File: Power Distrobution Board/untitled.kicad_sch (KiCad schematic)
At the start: 4 parts, among them J3 0768250004, K3 AZ2150-1A-12DEF

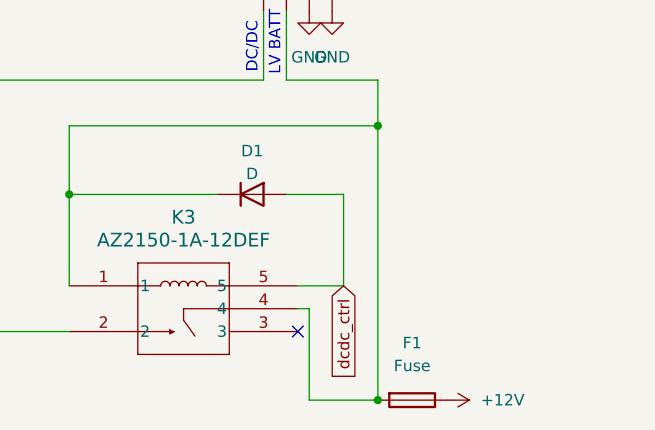
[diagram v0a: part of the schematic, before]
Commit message: changes after cdr
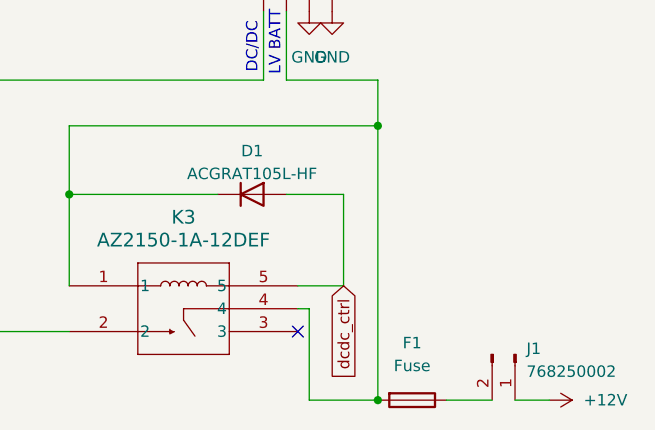
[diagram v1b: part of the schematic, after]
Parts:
- added J1: 768250002, Connector_Molex:Molex_Mega-Fit_76825-0002_2x01_P5.70mm_Horizontal, symbol Connector:Conn_01x02_Pin
- D1: value D -> ACGRAT105L-HF
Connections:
- net +12V: now also J1.1 (Pin_1); no longer F1.1
- new net: F1.1, J1.2 (Pin_2)
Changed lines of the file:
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@@
+	(wire
+		(pts
+			(xy 74.93 74.93) (xy 80.01 74.93)
+		)
+		(stroke
+			(width 0)
+			(type default)
+		)
+	)
 	(wire
 		(pts
@@
 		(pts
 			(xy 59.69 74.93) (xy 67.31 74.93)
+		)
+		(stroke
+			(width 0)
+			(type default)
+		)
+	)
+	(wire
+		(pts
+			(xy 82.55 74.93) (xy 86.36 74.93)
 		)
 		(stroke
@@
 		)
 	)
+	(netclass_flag ""
+		(length 2.54)
+		(shape round)
+		(at 77.47 74.93 180)
+		(fields_autoplaced yes)
+		(effects
+			(font
+				(size 1.27 1.27)
+			)
+			(justify right bottom)
+		)
+		(property "Netclass" "20a"
+			(at 78.1685 77.47 0)
+			(effects
+				(font
+					(size 1.27 1.27)
+					(italic yes)
+				)
+				(justify left)
+			)
+		)
+	)
 	(symbol
 		(lib_id "power:GND")
@@
 	)
 	(symbol
+		(lib_id "Connector:Conn_01x02_Pin")
+		(at 82.55 69.85 270)
+		(unit 1)
+		(exclude_from_sim no)
+		(in_bom yes)
+		(on_board yes)
+		(dnp no)
+		(fields_autoplaced yes)
+		(property "Reference" "J1"
+			(at 83.82 69.2149 90)
+			(effects
+				(font
+					(size 1.27 1.27)
+				)
+				(justify left)
+			)
+		)
+		(property "Value" "768250002"
+			(at 83.82 71.7549 90)
+			(effects
+				(font
+					(size 1.27 1.27)
+				)
+				(justify left)
+			)
+		)
+		(property "Footprint" "Connector_Molex:Molex_Mega-Fit_76825-0002_2x01_P5.70mm_Horizontal"
+			(at 82.55 69.85 0)
+			(effects
+				(font
+					(size 1.27 1.27)
+				)
+				(hide yes)
+			)
+		)
+		(property "Datasheet" "https://mm.digikey.com/Volume0/opasdata/d220001/medias/docus/1100/Mega-Fit_Power_Conn.pdf"
+			(at 82.55 69.85 0)
+			(effects
+				(font
+					(size 1.27 1.27)
+				)
+				(hide yes)
+			)
+		)
+		(property "Description" "Generic connector, single row, 01x02, script generated"
+			(at 82.55 69.85 0)
+			(effects
+				(font
+					(size 1.27 1.27)
+				)
+				(hide yes)
+			)
+		)
+		(pin "2"
+		)
+		(pin "1"
+		)
+		(instances
+			(project ""
+				(path "/cd827802-ab32-49ad-ad84-bccf81c569e7/5e60819f-ad8d-4ea9-981f-2629d0d45dd9"
+					(reference "J1")
+					(unit 1)
+				)
+			)
+		)
+	)
+	(symbol
 		(lib_id "AZ2150:AZ2150-1A-12DEF")
 		(at 33.02 62.23 0)
@@
 			)
 		)
-		(property "Value" "D"
+		(property "Value" "ACGRAT105L-HF"
 			(at 53.34 49.784 0)
 			(effects
@@
 	(symbol
 		(lib_id "power:+12V")
-		(at 74.93 74.93 270)
+		(at 86.36 74.93 270)
 		(unit 1)
 		(exclude_from_sim no)
@@
 		(fields_autoplaced yes)
 		(property "Reference" "#PWR07"
-			(at 71.12 74.93 0)
+			(at 82.55 74.93 0)
 			(effects
 				(font
@@
 		)
 		(property "Value" "+12V"
-			(at 78.74 74.9299 90)
+			(at 90.17 74.9299 90)
 			(effects
 				(font
@@
 		)
 		(property "Footprint" ""
-			(at 74.93 74.93 0)
+			(at 86.36 74.93 0)
 			(effects
 				(font
@@
 		)
 		(property "Datasheet" ""
-			(at 74.93 74.93 0)
+			(at 86.36 74.93 0)
 			(effects
 				(font
@@
 		)
 		(property "Description" "Power symbol creates a global label with name \"+12V\""
-			(at 74.93 74.93 0)
-			(effects
-				(font
+			(at 86.36 74.93 0)
+			(effects
+				(font

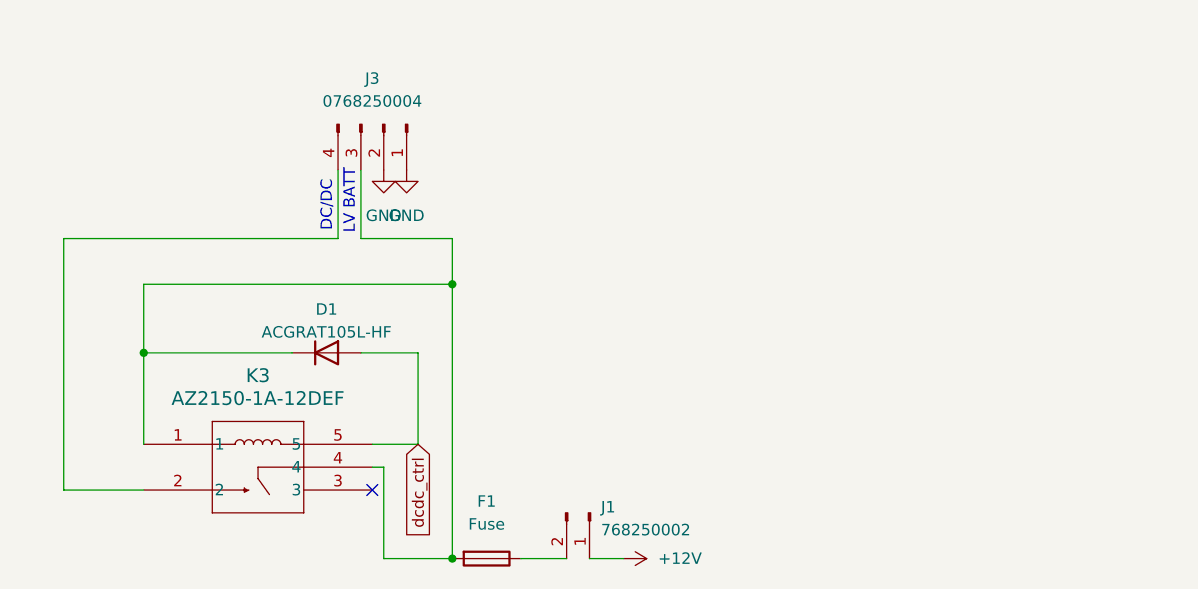
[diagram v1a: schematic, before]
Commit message: even newer changes
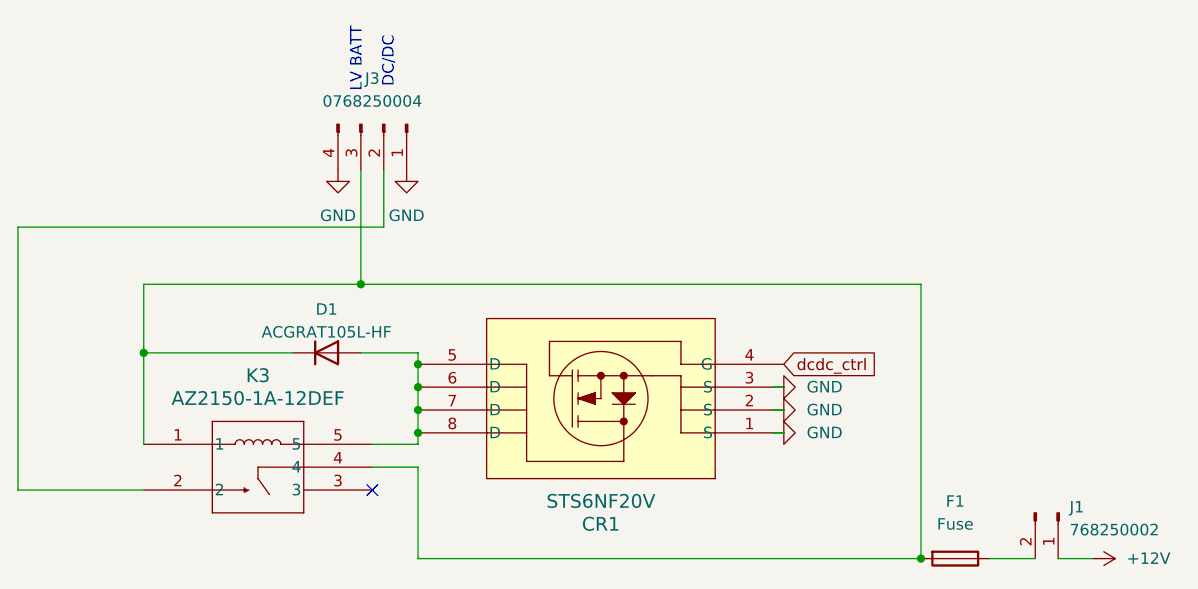
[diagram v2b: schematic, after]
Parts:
- added CR1: STS6NF20V, Package_SO:SOIC-8_3.9x4.9mm_P1.27mm, symbol FS_3_Global_Symbol_Library:STS6NF20V
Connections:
- net GND: now also J3.4 (Pin_4), CR1.1 (S), CR1.2 (S), CR1.3 (S); no longer J3.2 (Pin_2)
- net dcdc_ctrl: now also CR1.4 (G); no longer D1.2 (A), K3.5
- net at K3.2: now also J3.2 (Pin_2); no longer J3.4 (Pin_4)
- new net: CR1.5 (D), CR1.6 (D), CR1.7 (D), CR1.8 (D), D1.2 (A), K3.5
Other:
- moved on the sheet: F1, J1

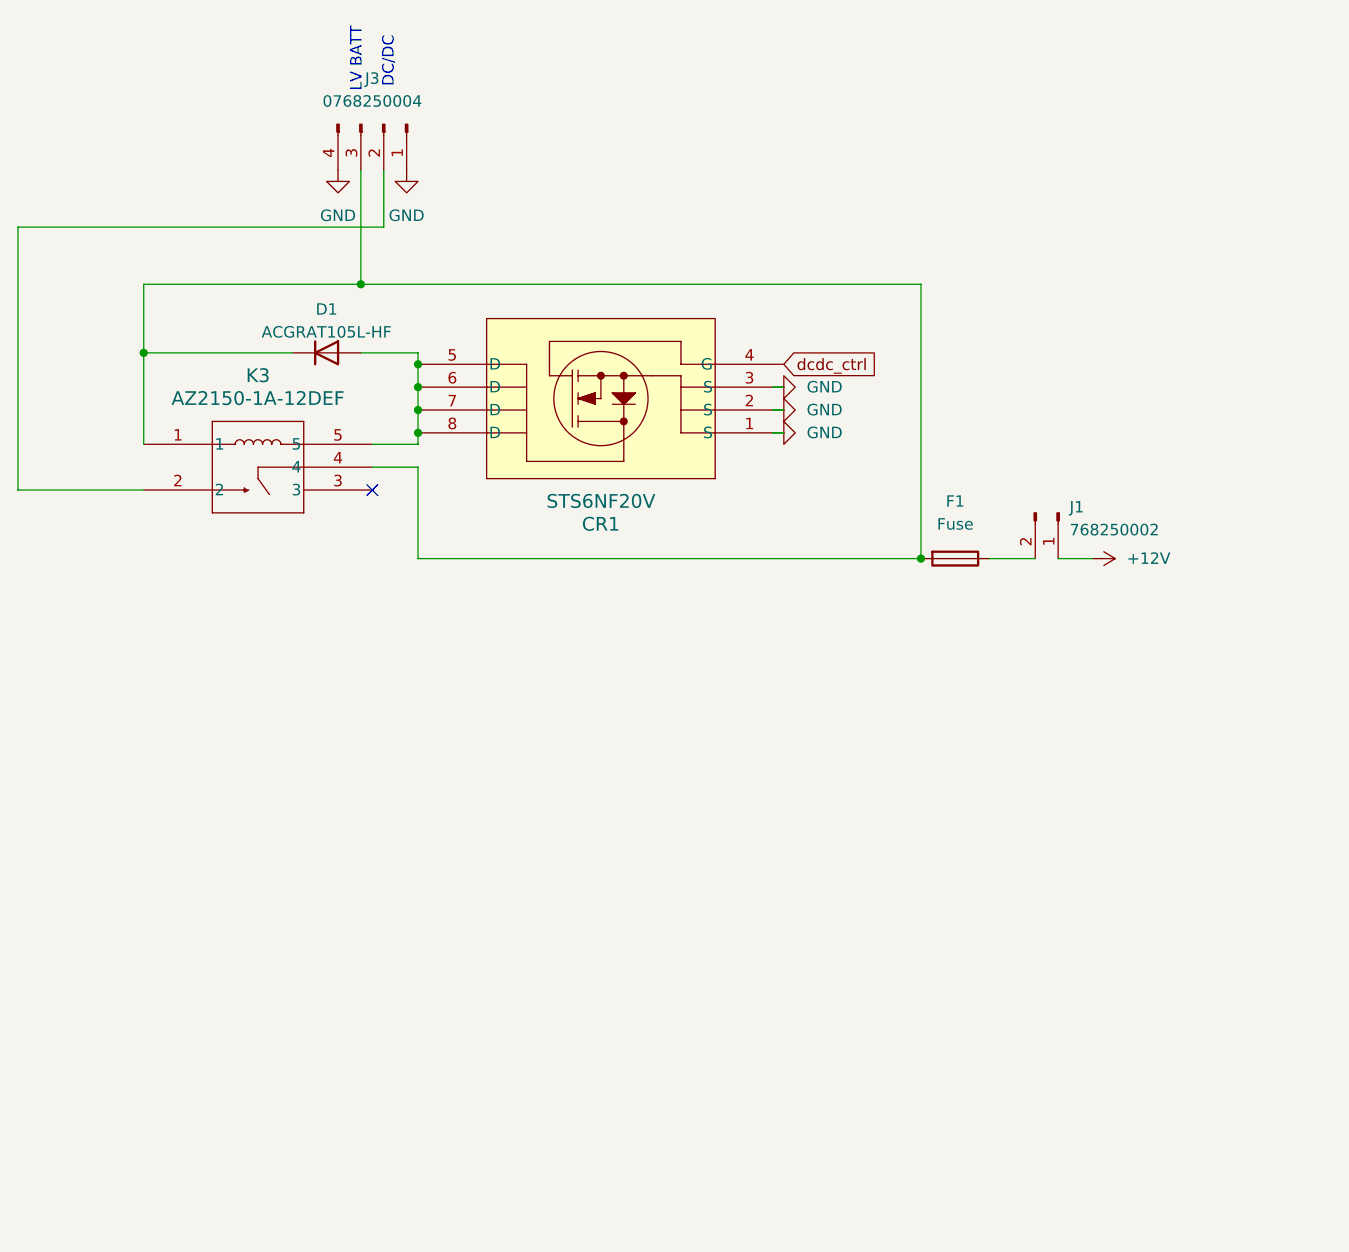
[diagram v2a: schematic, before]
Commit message: commit 1 of v2
pd board v2 work first commit
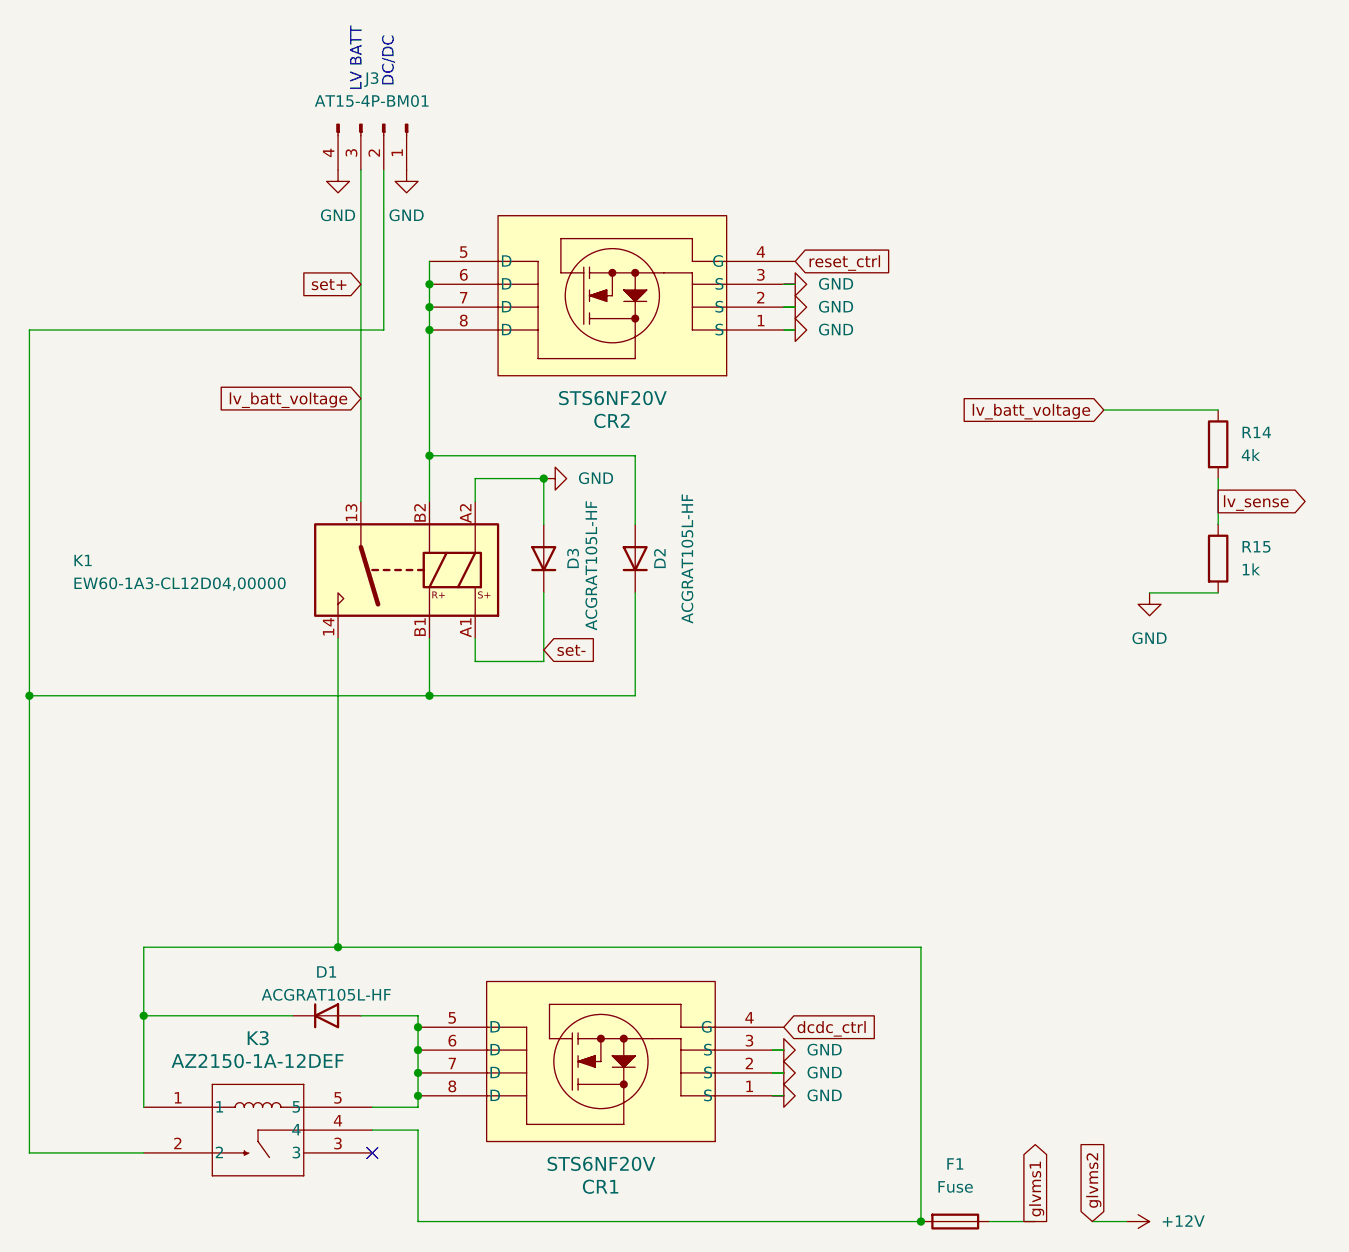
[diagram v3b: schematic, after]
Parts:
- removed J1: 768250002, Connector_Molex:Molex_Mega-Fit_76825-0002_2x01_P5.70mm_Horizontal, symbol Connector:Conn_01x02_Pin
- added CR2: STS6NF20V, Package_SO:SOIC-8_3.9x4.9mm_P1.27mm, symbol FS_3_Global_Symbol_Library:STS6NF20V
- added D2, D3: ACGRAT105L-HF, Diode_SMD:D_2010_5025Metric_Pad1.52x2.65mm_HandSolder, symbol Device:D
- added K1: EW60-1A3-CL12D04,00000, symbol Relay:Relay_SPST_Latching_2coil
- added R14: 4k, Resistor_SMD:R_0805_2012Metric_Pad1.20x1.40mm_HandSolder, symbol Device:R
- added R15: 1k, Resistor_SMD:R_0805_2012Metric_Pad1.20x1.40mm_HandSolder, symbol Device:R
- J3: value 0768250004 -> AT15-4P-BM01; footprint Connector_Molex:Molex_Mega-Fit_76825-0004_2x02_P5.70mm_Horizontal -> FS_3_Global_Footprint_Library:CONN4_DT15-4P-G003
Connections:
- net GND: now also CR2.1 (S), CR2.2 (S), CR2.3 (S), D3.2 (A), K1.A2, R15.2
- net glvms1: now reaches F1.1
- net at D1.1 (K), F1.2, K3.1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: now also K1.14; no longer J3.3 (Pin_3)
- net at J3.2 (Pin_2), K3.2: now also D2.1 (K), K1.B1
- new net: CR2.5 (D), CR2.6 (D), CR2.7 (D), CR2.8 (D), D2.2 (A), K1.B2
- new net lv_batt_voltage: J3.3 (Pin_3), K1.13, R14.1
- new net lv_sense: R14.2, R15.1
- new net reset_ctrl: CR2.4 (G)
- new net set-: D3.1 (K), K1.A1
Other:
- moved on the sheet: CR1, D1, F1, K3

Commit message: v2 3/29
almost done need to add mounting holes text, clean up screen printing, and get linear regs re speced
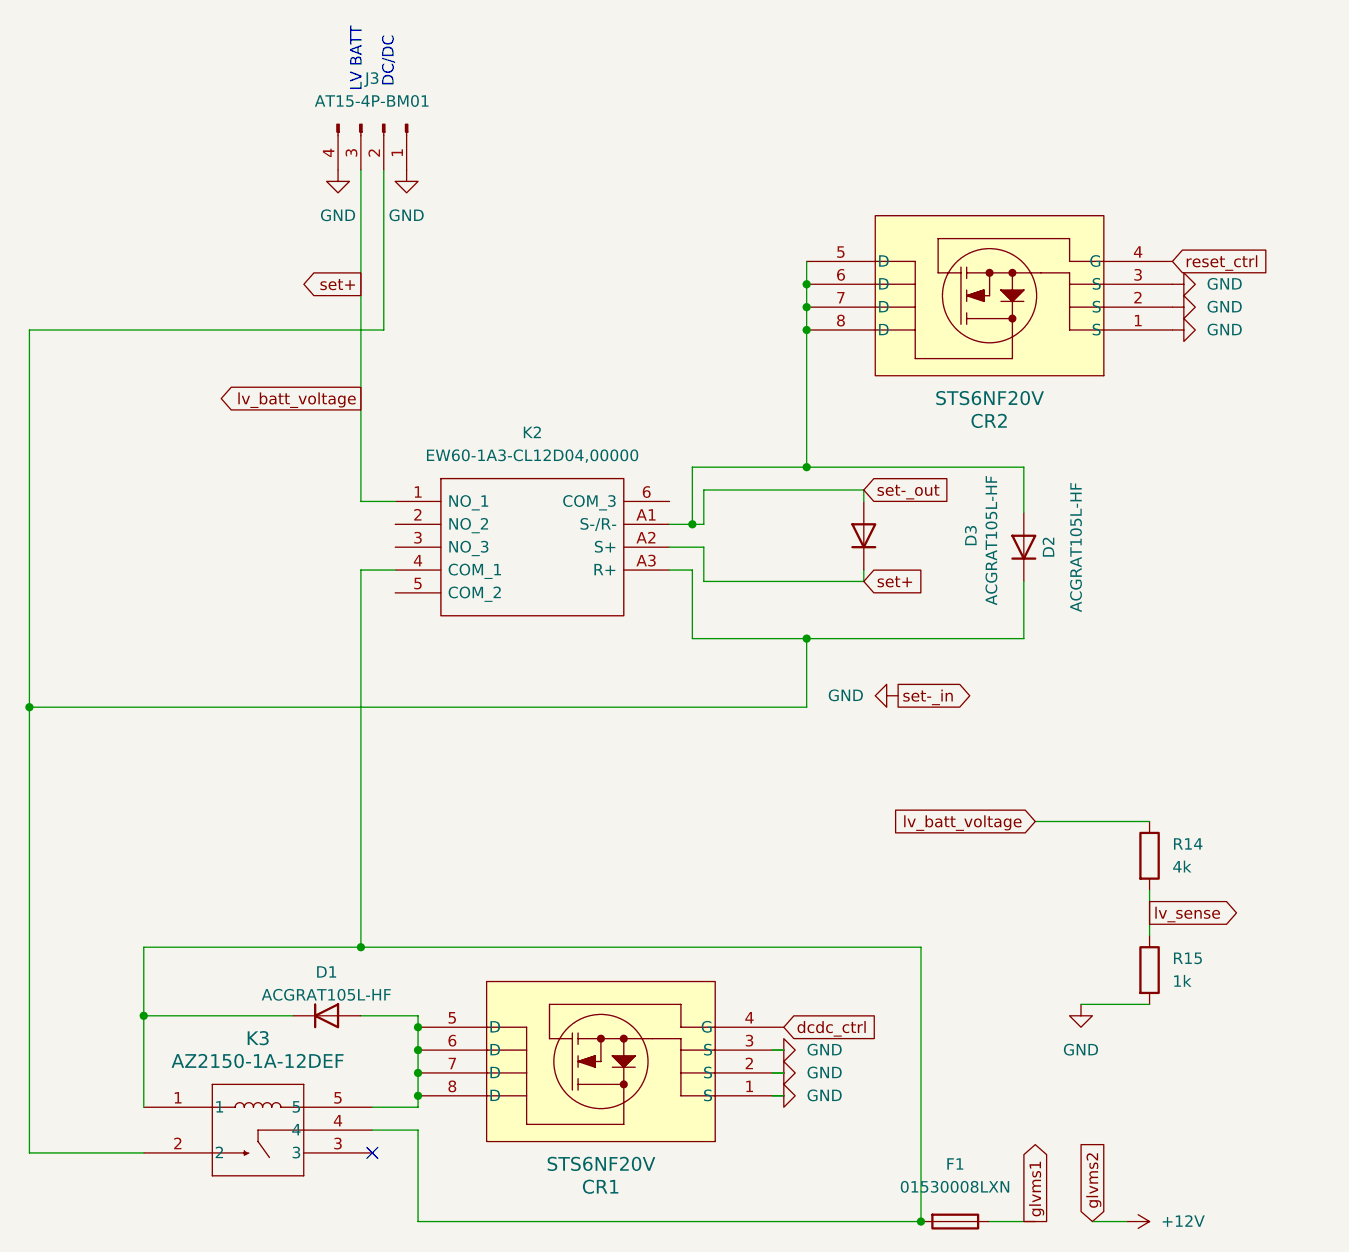
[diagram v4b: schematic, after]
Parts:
- removed K1: EW60-1A3-CL12D04,00000, symbol Relay:Relay_SPST_Latching_2coil
- added K2: EW60-1A3-CL12D04,00000, EW601A3CL12D0400000, symbol FS_3_Global_Symbol_Library:EW60-1A3-CL12D04,00000
- F1: value Fuse -> 01530008LXN; footprint project lib:CNM-03-BT mini blade fuse holder -> FS_3_Global_Footprint_Library:01530008LXN
- K3: footprint AZ2150_AMZ -> FS_3_Global_Footprint_Library:AZ2150_AMZ
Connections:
- net set- is gone; now on net lv_batt_voltage: D3.1 (K)
- net GND: no longer D3.2 (A)
- net lv_batt_voltage: now also K2.1 (NO_1), K2.A2 (S+)
- net set-_out: now reaches CR2.5 (D), CR2.6 (D), CR2.7 (D), CR2.8 (D), D2.2 (A)
- net set-_out: now also D3.2 (A), K2.A1 (S-/R-)
- net at D2.1 (K), J3.2 (Pin_2), K3.2: now also K2.A3 (R+)
- net at D1.1 (K), F1.2, K3.1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: now also K2.4 (COM_1)
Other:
- moved on the sheet: CR2, R14, R15
